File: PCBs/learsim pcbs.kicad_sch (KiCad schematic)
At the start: 58 parts, among them SW1 MHz, SW2 KHz, SW3 2MD1T1B1M2QES-5, U1 ESP32-C6-DEV-KIT-N8, U2 MAX7219, U3 MAX7219

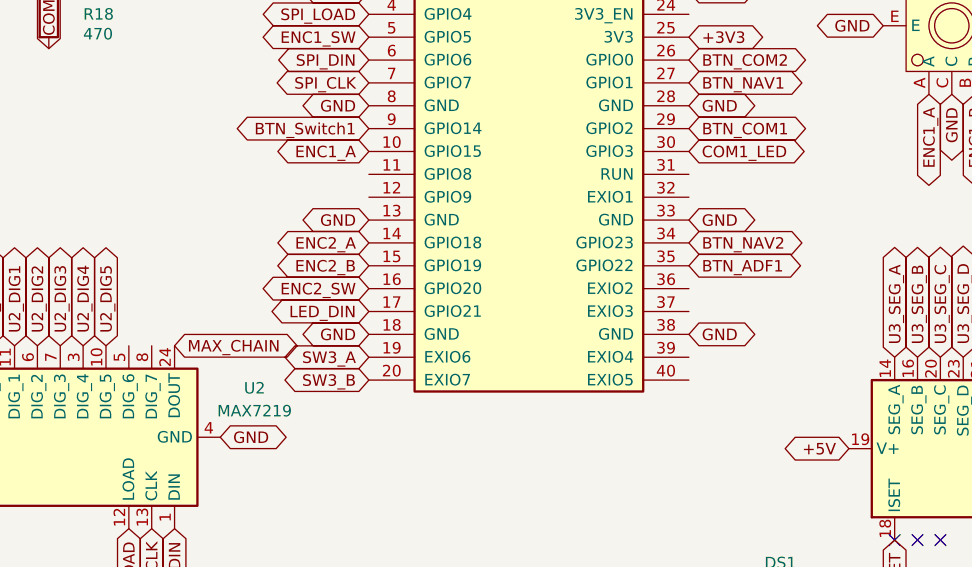
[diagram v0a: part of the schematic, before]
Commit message: v1.0
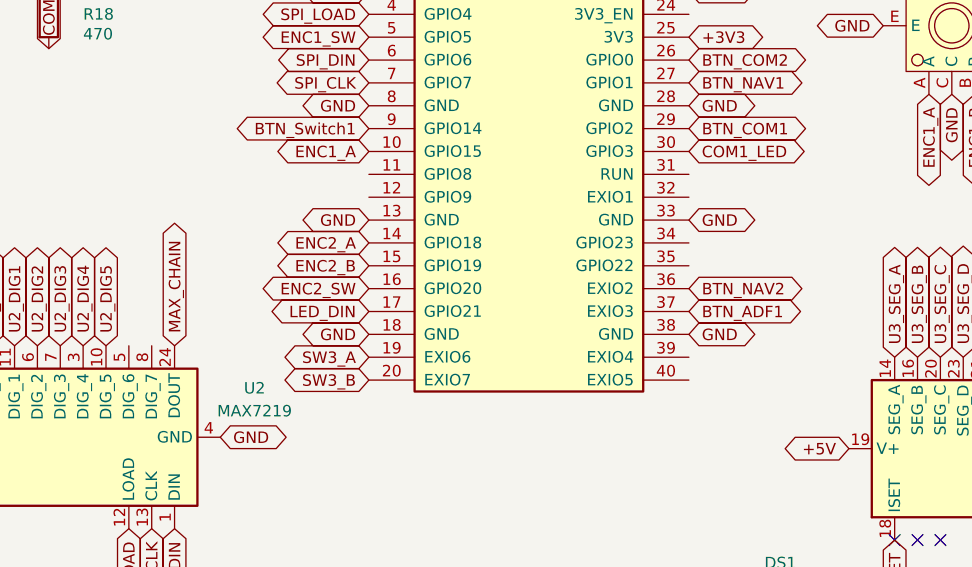
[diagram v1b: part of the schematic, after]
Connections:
- net BTN_ADF1: now also U1.37 (EXIO3); no longer U1.35 (GPIO22)
- net BTN_NAV2: now also U1.36 (EXIO2); no longer U1.34 (GPIO23)
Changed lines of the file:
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@@
 	(global_label "BTN_NAV2"
 		(shape bidirectional)
-		(at 147.32 114.3 0)
-		(fields_autoplaced yes)
-		(effects
-			(font
-				(size 1.27 1.27)
-			)
-			(justify left)
-		)
-		(property "Intersheetrefs" "${INTERSHEET_REFS}"
-			(at 160.1856 114.3 0)
+		(at 147.32 119.38 0)
+		(fields_autoplaced yes)
+		(effects
+			(font
+				(size 1.27 1.27)
+			)
+			(justify left)
+		)
+		(property "Intersheetrefs" "${INTERSHEET_REFS}"
+			(at 160.1856 119.38 0)
 			(hide yes)
 			(show_name no)
@@
 	(global_label "BTN_ADF1"
 		(shape bidirectional)
-		(at 147.32 116.84 0)
-		(fields_autoplaced yes)
-		(effects
-			(font
-				(size 1.27 1.27)
-			)
-			(justify left)
-		)
-		(property "Intersheetrefs" "${INTERSHEET_REFS}"
-			(at 160.1856 116.84 0)
+		(at 147.32 121.92 0)
+		(fields_autoplaced yes)
+		(effects
+			(font
+				(size 1.27 1.27)
+			)
+			(justify left)
+		)
+		(property "Intersheetrefs" "${INTERSHEET_REFS}"
+			(at 160.1856 121.92 0)
 			(hide yes)
 			(show_name no)
@@
 	(global_label "MAX_CHAIN"
 		(shape bidirectional)
-		(at 90.17 125.73 0)
-		(fields_autoplaced yes)
-		(effects
-			(font
-				(size 1.27 1.27)
-			)
-			(justify left)
-		)
-		(property "Intersheetrefs" "${INTERSHEET_REFS}"
-			(at 104.608 125.73 0)
-			(hide yes)
-			(show_name no)
+		(at 90.17 125.73 90)
+		(fields_autoplaced yes)
+		(effects
+			(font
+				(size 1.27 1.27)
+			)
+			(justify left)
+		)
+		(property "Intersheetrefs" "${INTERSHEET_REFS}"
+			(at 90.17 111.292 90)
+			(hide yes)
+			(show_name no)
